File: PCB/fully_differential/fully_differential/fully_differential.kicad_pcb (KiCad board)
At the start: 2 copper layers, 38 parts, among them U1 LM741, U2 LM741, U3 LM741, U4 LM741, U5 LM324, U6 AD8138, U7 LM324

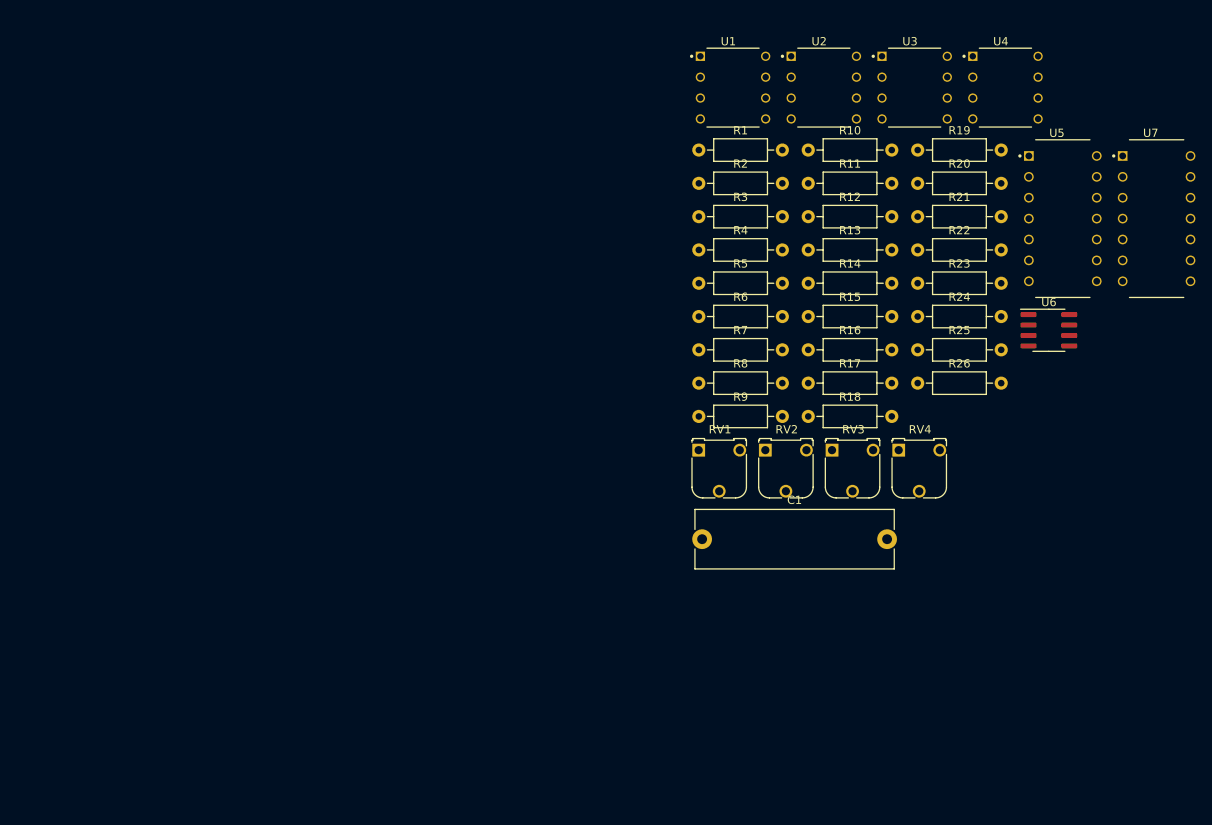
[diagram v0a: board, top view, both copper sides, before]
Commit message: new pcb
falta validar para impressao
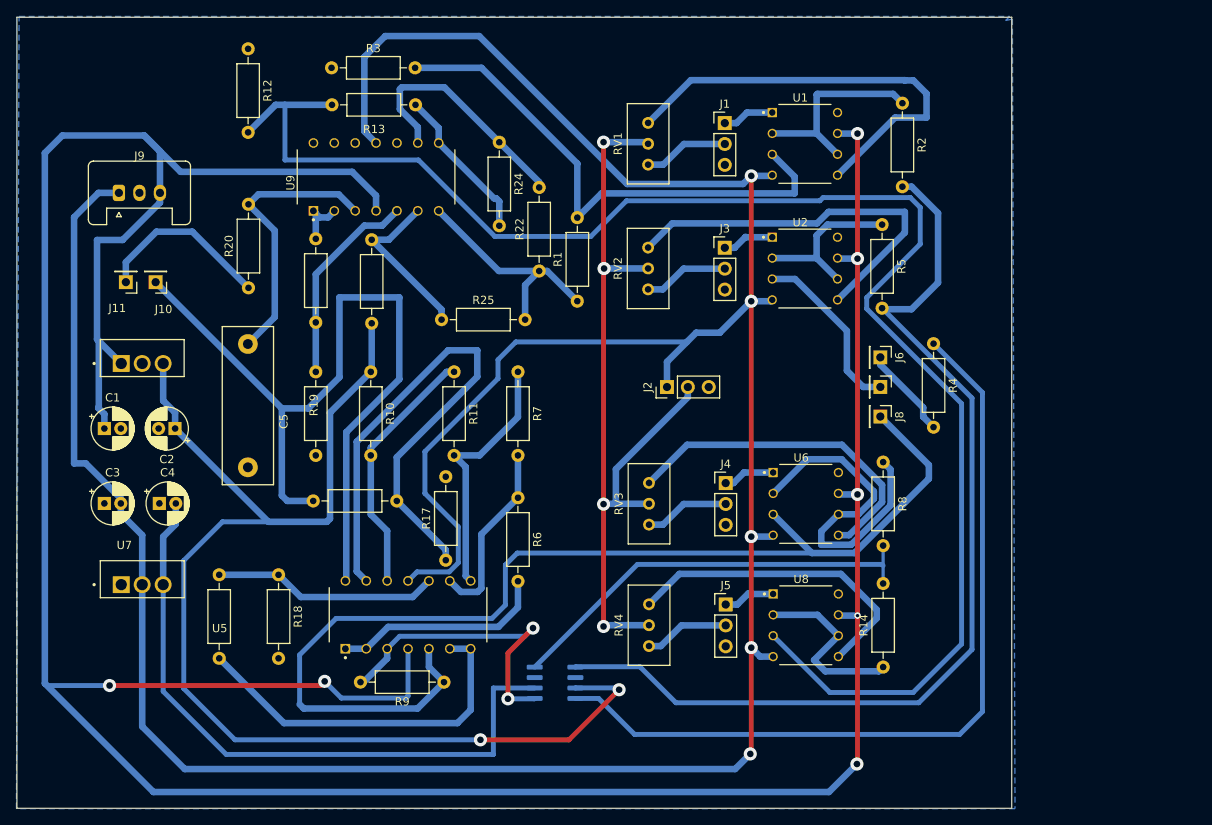
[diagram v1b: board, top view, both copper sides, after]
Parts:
- removed R26: R, Resistor_THT:R_Axial_DIN0207_L6.3mm_D2.5mm_P10.16mm_Horizontal
- added C2: C, Capacitor_THT:CP_Radial_D5.0mm_P2.00mm, F.Cu at (52.9, 107.9)
- added C3: C, Capacitor_THT:CP_Radial_D5.0mm_P2.00mm, F.Cu at (44.3, 117.0)
- added C4: C, Capacitor_THT:CP_Radial_D5.0mm_P2.00mm, F.Cu at (51.0, 117.0)
- added C5: C, Capacitor_THT:C_Rect_L19.0mm_W6.0mm_P15.00mm_MKS4, F.Cu at (61.8, 97.7)
- added J1: Conn_01x03, Connector_PinHeader_2.54mm:PinHeader_1x03_P2.54mm_Vertical, F.Cu at (119.8, 70.8)
- added J10: PIN_A0, Connector_PinHeader_2.54mm:PinHeader_1x01_P2.54mm_Vertical, F.Cu at (50.6, 90.1)
- added J11: PIN_09, Connector_PinHeader_2.54mm:PinHeader_1x01_P2.54mm_Vertical, F.Cu at (46.9, 90.1)
- added J2: Conn_01x03, Connector_PinHeader_2.54mm:PinHeader_1x03_P2.54mm_Vertical, F.Cu at (112.8, 102.9)
- added J3: Conn_01x03, Connector_PinHeader_2.54mm:PinHeader_1x03_P2.54mm_Vertical, F.Cu at (119.8, 86.0)
- added J4: Conn_01x03, Connector_PinHeader_2.54mm:PinHeader_1x03_P2.54mm_Vertical, F.Cu at (119.9, 114.6)
- added J5: Conn_01x03, Connector_PinHeader_2.54mm:PinHeader_1x03_P2.54mm_Vertical, F.Cu at (119.9, 129.3)
- added J6: Conn_01x01, Connector_PinHeader_2.54mm:PinHeader_1x01_P2.54mm_Vertical, F.Cu at (138.7, 99.3)
- added J7: Conn_01x01, Connector_PinHeader_2.54mm:PinHeader_1x01_P2.54mm_Vertical, F.Cu at (138.7, 102.9)
- added J8: Conn_01x01, Connector_PinHeader_2.54mm:PinHeader_1x01_P2.54mm_Vertical, F.Cu at (138.7, 106.5)
- added J9: Conn_01x03, Connector_Stocko:Stocko_MKS_1653-6-0-303_1x3_P2.50mm_Vertical, F.Cu at (46.1, 79.3)
- added U8: LM741, lm741:DIP794W45P254L959H508Q8, F.Cu at (129.6, 131.9)
- added U9: LM324, lm324:DIP825W47P254L1917H533Q14, F.Cu at (77.4, 77.3)
- C1: footprint Capacitor_THT:C_Rect_L24.0mm_W7.0mm_P22.50mm_MKT -> Capacitor_THT:CP_Radial_D5.0mm_P2.00mm
- RV1, RV2, RV3, RV4: footprint Potentiometer_THT:Potentiometer_Runtron_RM-065_Vertical -> Potentiometer_THT:Potentiometer_Bourns_3296W_Vertical
- U3: value LM741 -> AD8138; footprint lm741:DIP794W45P254L959H508Q8 -> Package_SO:SOIC-8_3.9x4.9mm_P1.27mm; moved to B.Cu
- U4: value LM741 -> L7805; footprint lm741:DIP794W45P254L959H508Q8 -> l7805:TO255P1020X450X2000-3
- U6: value AD8138 -> LM741; footprint Package_SO:SOIC-8_3.9x4.9mm_P1.27mm -> lm741:DIP794W45P254L959H508Q8
- U7: value LM324 -> L7905; footprint lm324:DIP825W47P254L1917H533Q14 -> l7805:TO255P1020X450X2000-3
- moved U7 130.9 mm to (48.9, 126.3)
- moved U4 110.0 mm to (48.9, 99.4)
- moved U5 93.1 mm to (81.3, 130.6), turned to 90 degrees
- moved U3 84.6 mm to (99.1, 138.9), turned to 180 degrees
- moved R20 82.4 mm to (61.9, 90.8), turned to 90 degrees
- moved R19 78.0 mm to (70.0, 101.0), turned to -90 degrees
- moved R16 76.7 mm to (58.3, 125.7), turned to -90 degrees
- moved C1 73.9 mm to (44.3, 107.9)
- moved R21 73.3 mm to (70.0, 84.9), turned to -90 degrees
- moved R12 71.1 mm to (61.8, 61.8), turned to -90 degrees
- moved R18 67.2 mm to (65.5, 125.7), turned to -90 degrees
- moved R23 66.6 mm to (76.8, 95.1), turned to 90 degrees
- moved R15 64.3 mm to (69.7, 116.7)
- moved R10 59.7 mm to (76.7, 101.0), turned to -90 degrees
- moved R25 58.0 mm to (85.3, 94.7)
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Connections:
- C1 pad 1: Net-(U5A-+) -> +9V
- R1 pad 1: Net-(U2-+) -> t+
- R10 pad 1: Net-(U4--) -> +5V
- R10 pad 2: Net-(U6--IN) -> Net-(U5D-+)
- R11 pad 1: Net-(U5A--) -> Net-(U5D-+)
- R11 pad 2: Net-(U5B-+) -> Net-(R11-Pad2)
- R12 pad 1: +5V -> GND
- R12 pad 2: Net-(U5B--) -> Net-(U8-+)
- R13 pad 1: Net-(U5B--) -> t-
- R13 pad 2: t+ -> Net-(U8-+)
- R14 pad 1: Net-(U5B-+) -> Net-(U8--)
- R14 pad 2: GND -> Net-(U3-+IN)
- R15 pad 1: Net-(U6-RANGE) -> Net-(J10-Pin_1)
- R15 pad 2: Net-(U1-+) -> Net-(U5D--)
- R16 pad 1: Net-(U2-+) -> Net-(U5C-+)
- R16 pad 2: Net-(U6-OUT) -> Net-(U5B--)
- R17 pad 1: t+ -> Net-(U5D--)
- R17 pad 2: Net-(U5C--) -> GND
- R18 pad 1: Net-(U5C--) -> Net-(U5C-+)
- R18 pad 2: t- -> GND
- R19 pad 1: Net-(U7C-+) -> Net-(U9B-+)
- R19 pad 2: Net-(U7B--) -> GND
- R2 pad 1: t- -> Net-(U1--)
- R2 pad 2: Net-(U3-+) -> Net-(U3--IN)
- R20 pad 1: Net-(U7C--) -> Net-(J11-Pin_1)
- R20 pad 2: Net-(U7A--) -> Net-(U9A-+)
- R21 pad 1: Net-(U7C-+) -> Net-(U9A--)
- R21 pad 2: GND -> Net-(U9B-+)
- R22 pad 1: Net-(R22-Pad1) -> t+
- R22 pad 2: Net-(U7C--) -> Net-(U9C--)
- R23 pad 1: Net-(U5D-+) -> +5V
- R23 pad 2: Net-(R22-Pad1) -> Net-(U9B--)
- R24 pad 1: +5V -> Net-(U9C--)
- R24 pad 2: Net-(U5D-+) -> t-
- R25 pad 1: Net-(U5D--) -> Net-(U9B--)
- R25 pad 2: GND -> t+
- R3 pad 1: t+ -> GND
- R3 pad 2: Net-(U4-+) -> Net-(U1-+)
- R4 pad 1: v+ -> Net-(U3-RANGE)
- R4 pad 2: Net-(U5A-+) -> Net-(J6-Pin_1)
- R5 pad 1: GND -> Net-(U2--)
- R5 pad 2: Net-(U4-+) -> Net-(U3--IN)
- R6 pad 1: GND -> Net-(U5C--)
- R6 pad 2: Net-(U3-+) -> Net-(U5A--)
- R7 pad 1: Net-(U2--) -> Net-(R11-Pad2)
- R7 pad 2: Net-(U6-+IN) -> Net-(U5C--)
- R8 pad 1: Net-(U1--) -> Net-(U6--)
- R8 pad 2: Net-(U6--IN) -> Net-(U3-+IN)
- R9 pad 1: Net-(U3--) -> Net-(J8-Pin_1)
- R9 pad 2: Net-(U6-+IN) -> Net-(U3-OUT)
- RV1 pad 2: -9V -> Net-(J2-Pin_2)
- RV1 pad 3: op1_1 -> Net-(J1-Pin_2)
- RV2 pad 2: -9V -> Net-(J2-Pin_2)
- RV2 pad 3: op2_1 -> Net-(J3-Pin_2)
- RV3 pad 2: -9V -> Net-(J2-Pin_2)
- RV3 pad 3: op3_1 -> Net-(J4-Pin_2)
- RV4 pad 2: -9V -> Net-(J2-Pin_2)
- RV4 pad 3: op4_1 -> Net-(J5-Pin_2)
- U1 pad 1: op2_1 -> op1_1
- U1 pad 5: op2_2 -> op1_2
- U2 pad 1: op3_1 -> op2_1
- U2 pad 3: Net-(U2-+) -> Net-(J7-Pin_1)
- U2 pad 5: op3_2 -> op2_2
- U3 pad 1: op4_1 -> Net-(U3--IN)
- U3 pad 2: Net-(U3--) -> unconnected-(U3-GND-Pad2)
- U3 pad 3: Net-(U3-+) -> +5V
- U3 pad 4: -9V -> Net-(U3-RANGE)
- U3 pad 5: op4_2 -> Net-(U3-OUT)
- U3 pad 6: Net-(U3--) -> -5V
- U3 pad 7: +9V -> unconnected-(U3-Vref1-Pad7)
- U3 pad 8: unconnected-(U3-NC-Pad8) -> Net-(U3-+IN)
- U4 pad 1: op1_1 -> +9V
- U4 pad 2: Net-(U4--) -> GND
- U4 pad 3: Net-(U4-+) -> +5V
- U5 pad 1: (no net) -> Net-(U5A--)
- U5 pad 10: (no net) -> Net-(U5C-+)
- U5 pad 11: (no net) -> -9V
- U5 pad 14: A0 -> Net-(J10-Pin_1)
- U5 pad 2: (no net) -> Net-(U5A--)
- U5 pad 3: (no net) -> Net-(U3-OUT)
- U5 pad 4: (no net) -> +9V
- U5 pad 5: (no net) -> Net-(J8-Pin_1)
- U5 pad 6: (no net) -> Net-(U5B--)
- U5 pad 7: (no net) -> Net-(U5B--)
- U5 pad 8: (no net) -> Net-(R11-Pad2)
- U5 pad 9: (no net) -> Net-(U5C--)
- U6 pad 1: Net-(U6--IN) -> op3_1
- U6 pad 2: unconnected-(U6-GND-Pad2) -> Net-(U6--)
- U6 pad 3: +5V -> Net-(J8-Pin_1)
- U6 pad 4: Net-(U6-RANGE) -> -9V
- U6 pad 5: Net-(U6-OUT) -> op3_2
- U6 pad 6: -5V -> Net-(U6--)
- U6 pad 7: unconnected-(U6-Vref1-Pad7) -> +9V
- U6 pad 8: Net-(U6-+IN) -> unconnected-(U6-NC-Pad8)
- U7 pad 1: Net-(U7A--) -> GND
- U7 pad 2: Net-(U7A--) -> -9V
- U7 pad 3: Net-(U6-OUT) -> -5V
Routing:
- net +9V: track 0.00 -> 399.5 mm, vias 0 -> 7
- net -9V: track 0.00 -> 375.5 mm, vias 0 -> 5
- net Net-(U8-+): track 0.00 -> 190.7 mm
- net +5V: track 0.00 -> 149.4 mm, vias 0 -> 2
- net Net-(J8-Pin_1): track 0.00 -> 134.9 mm
- net Net-(U3--IN): track 0.00 -> 121.2 mm
- net Net-(U3-RANGE): track 0.00 -> 99.7 mm
- net Net-(J2-Pin_2): track 0.00 -> 99.3 mm, vias 0 -> 4
- net Net-(J10-Pin_1): track 0.00 -> 99.2 mm
- net -5V: track 0.00 -> 79.9 mm
- net Net-(U5D--): track 0.00 -> 68.7 mm
- net Net-(U1-+): track 0.00 -> 64.7 mm
- net op1_2: track 0.00 -> 53.4 mm
- net Net-(U3-+IN): track 0.00 -> 51.5 mm
- net op2_2: track 0.00 -> 47.1 mm
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- added copper zone on B.Cu, net GND
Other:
- board outline added: 121 x 96.2 mm
